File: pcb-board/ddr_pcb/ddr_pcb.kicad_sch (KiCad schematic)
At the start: 1 part, among them U1 RP2040_Zero

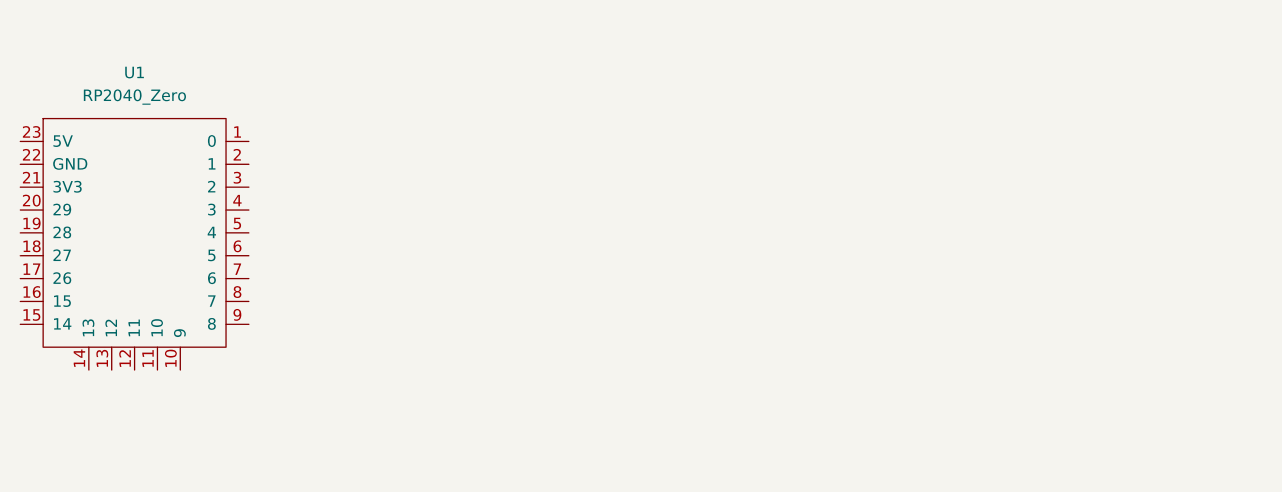
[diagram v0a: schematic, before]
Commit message: yay update
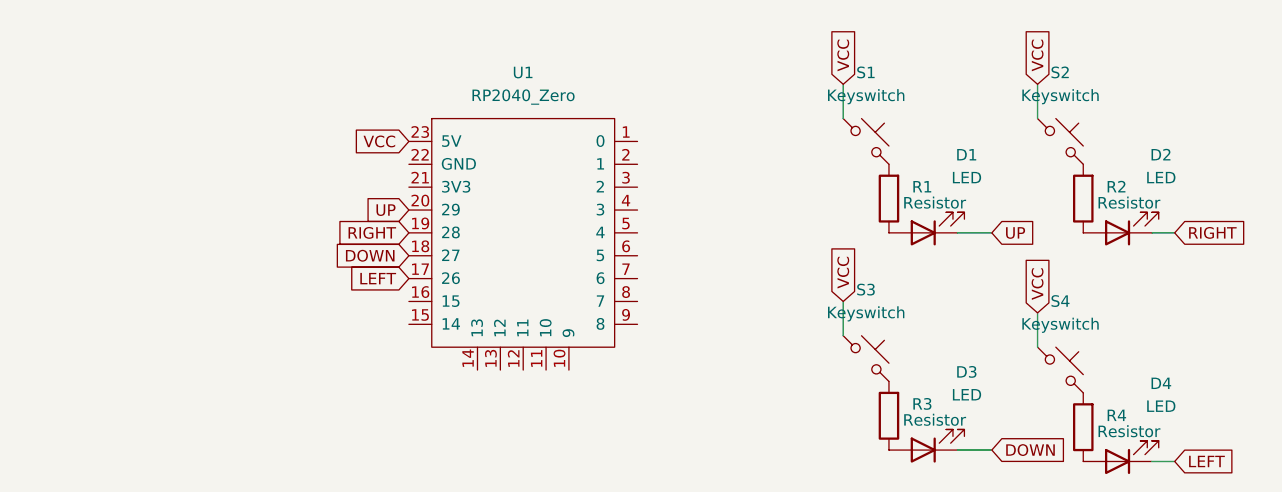
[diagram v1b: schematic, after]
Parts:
- added D1, D2, D3, D4: LED, LED_THT:LED_D1.8mm_W1.8mm_H2.4mm_Horizontal_O1.27mm_Z1.6mm, symbol Device:LED
- added R1, R2, R3, R4: Resistor, Resistor_THT:R_Axial_DIN0207_L6.3mm_D2.5mm_P10.16mm_Horizontal, symbol ScottoKeebs:Placeholder_Resistor
- added S1, S2, S3, S4: Keyswitch, ScottoKeebs_Choc:Choc_V1, symbol ScottoKeebs:Placeholder_Keyswitch
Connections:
- net LEFT: now reaches U1.17 (26)
- net LEFT: now also D4.1 (K)
- net DOWN: now reaches U1.18 (27)
- net DOWN: now also D3.1 (K)
- net RIGHT: now reaches U1.19 (28)
- net RIGHT: now also D2.1 (K)
- net UP: now reaches U1.20 (29)
- net UP: now also D1.1 (K)
- net VCC: now reaches U1.23 (5V)
- net VCC: now also S1.1, S2.1, S3.1, S4.1
- new net: R2.2, S2.2
- new net: R3.2, S3.2
- new net: D3.2 (A), R3.1
- new net: D2.2 (A), R2.1
- new net: D1.2 (A), R1.1
- new net: R1.2, S1.2
- new net: D4.2 (A), R4.1
- new net: R4.2, S4.2
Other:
- moved on the sheet: U1
